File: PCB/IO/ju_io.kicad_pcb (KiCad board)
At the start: 2 copper layers, 30 x 65 mm, 17 parts, among them J1 Conn_01x05, J2 Conn_01x05, J3 Conn_01x05, J4 Conn_01x05, J5 Conn_01x03, J6 Conn_01x03, U1 PiPico_No_SWD

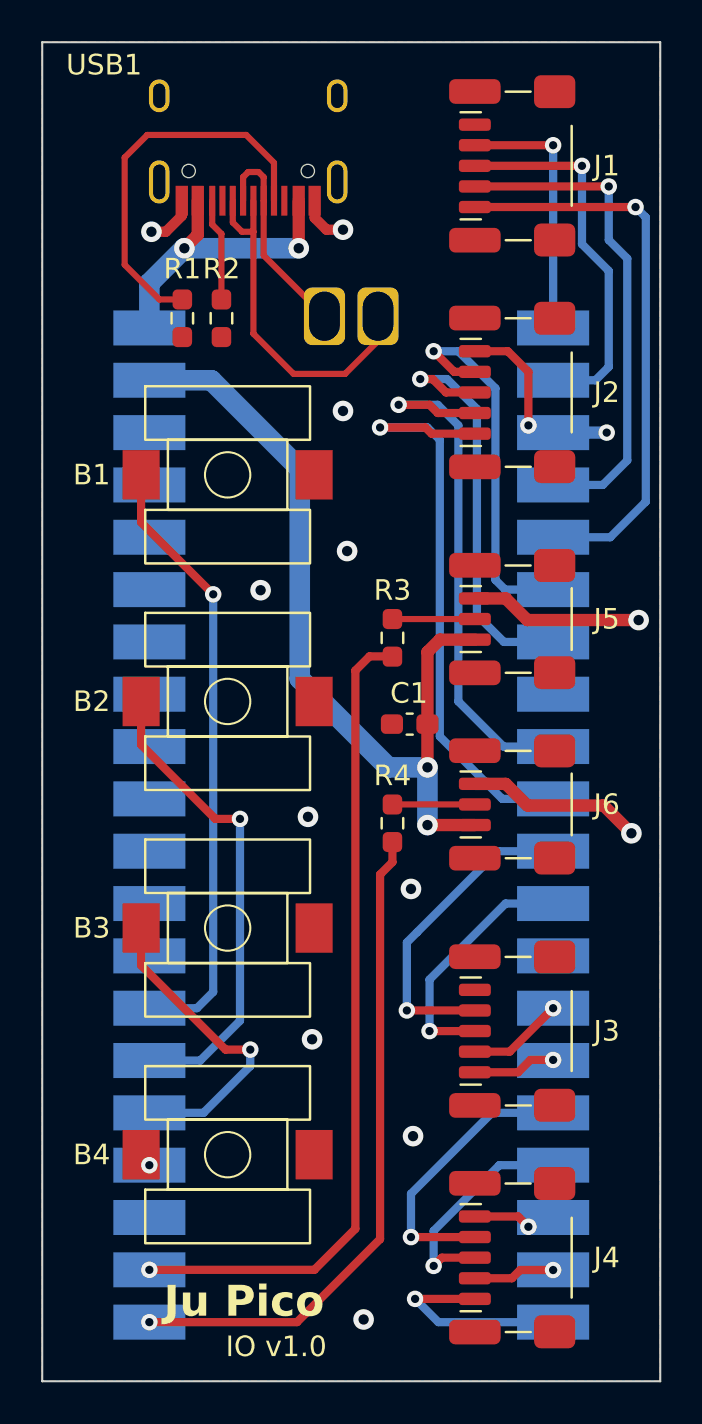
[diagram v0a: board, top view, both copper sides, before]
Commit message: PCBs of v1.1
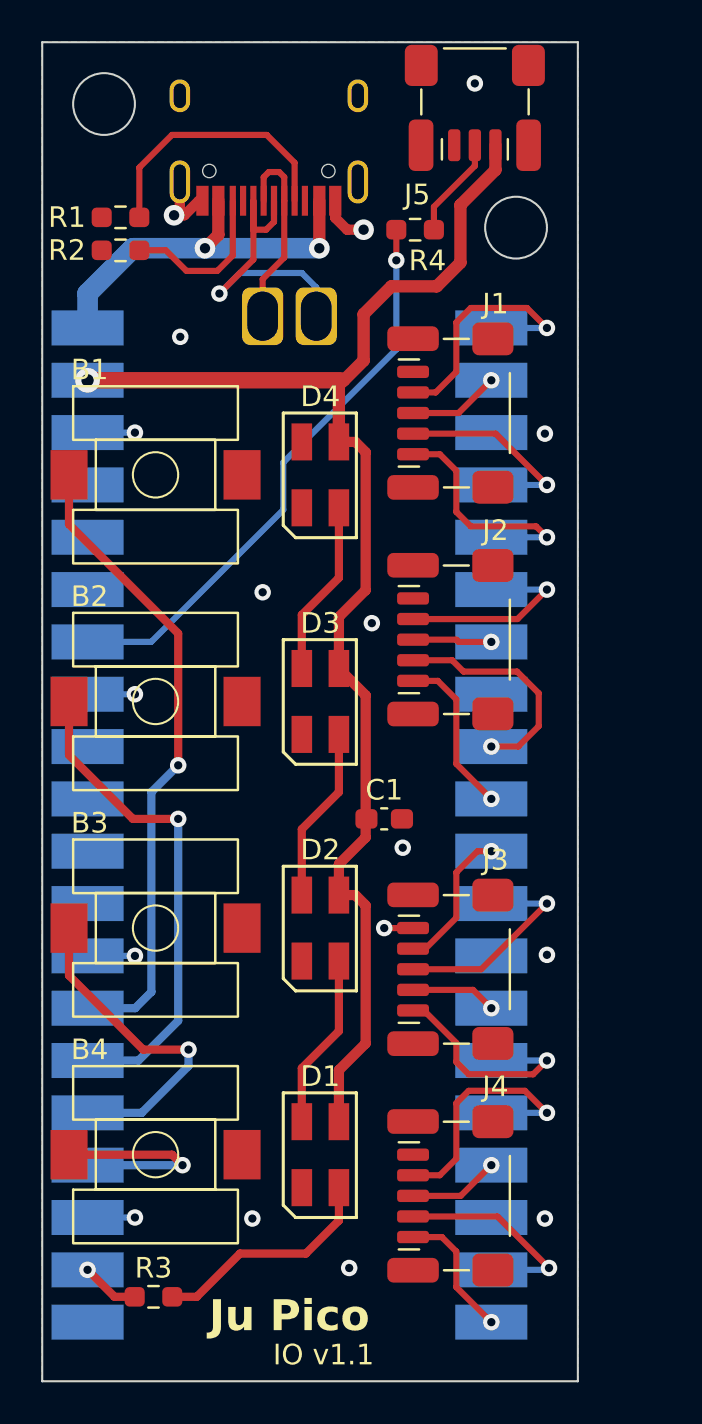
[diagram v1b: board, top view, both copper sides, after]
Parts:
- removed J6: Conn_01x03, ju_io:SH1.0_3P
- added D1: WS2812B_Unified, ju_io:WS2812B-2835, F.Cu at (138.6, 121.7)
- added D2: WS2812B_Unified, ju_io:WS2812B-2835, F.Cu at (138.6, 110.7)
- added D3: WS2812B_Unified, ju_io:WS2812B-2835, F.Cu at (138.6, 99.7)
- added D4: WS2812B_Unified, ju_io:WS2812B-2835, F.Cu at (138.6, 88.7)
- U1: footprint ju_io:RPi_Pico_SMD_Pins_No_SWD -> ju_io:RPi_Pico_SMD_Pins_No_SWD_No_Text
- moved R3 34.0 mm to (130.5, 128.6), turned to 0 degrees
- moved R4 28.8 mm to (143.2, 76.8), turned to 0 degrees
- moved J5 25.1 mm to (146.1, 70.7), turned to 180 degrees
- moved J1 12.4 mm to (145.1, 85.7)
- moved J2 12.4 mm to (145.1, 96.7)
- moved R2 5.91 mm to (128.9, 77.8), turned to 180 degrees
- moved R1 5.75 mm to (128.9, 76.2), turned to 180 degrees
- moved C1 4.76 mm to (141.7, 105.4), turned to 0 degrees
- moved J3 4.24 mm to (145.1, 112.7)
- moved J4 4.24 mm to (145.1, 123.7)
- moved B1 3.50 mm to (130.6, 88.7)
- moved B2 3.50 mm to (130.6, 99.7)
- moved B3 3.50 mm to (130.6, 110.7)
- moved B4 3.50 mm to (130.6, 121.7)
- moved U1 3.00 mm to (137.1, 105.7)
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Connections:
- R3 pad 2: Net-(J5-Pin_2) -> Net-(D1-In)
- R4 pad 1: Net-(U1-GPIO16) -> Net-(U1-GPIO28_ADC2)
- R4 pad 2: Net-(J6-Pin_2) -> Net-(J5-Pin_2)
- U1 pad 21: Net-(U1-GPIO16) -> unconnected-(U1-GPIO16-Pad21)
- U1 pad 34: unconnected-(U1-GPIO28_ADC2-Pad34) -> Net-(U1-GPIO28_ADC2)
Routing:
- net Net-(U1-GPIO17): track 40.0 -> 2.83 mm
- net Net-(U1-GPIO16): track 32.4 -> 0.00 mm, vias 1 -> 0
- net Net-(U1-GPIO28_ADC2): track 0.00 -> 28.0 mm, vias 0 -> 1
- net +5V: track 40.5 -> 68.4 mm, vias 2 -> 1
- net Net-(J2-Pin_1): track 29.0 -> 8.01 mm
- net Net-(J2-Pin_3): track 20.5 -> 3.85 mm
- net GND: track 33.0 -> 16.4 mm, vias 15 -> 17
- net Net-(J1-Pin_1): track 27.5 -> 12.0 mm
- net Net-(J2-Pin_2): track 26.1 -> 11.1 mm
- net Net-(J1-Pin_2): track 24.3 -> 10.2 mm
- net Net-(J1-Pin_3): track 18.5 -> 4.46 mm
- net Net-(D1-In): track 0.00 -> 11.2 mm
- net Net-(B4-A): track 0.00 -> 10.3 mm
- net Net-(J2-Pin_4): track 18.5 -> 9.79 mm
- net Net-(D3-Out): track 0.00 -> 8.55 mm
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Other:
- board size 30 x 65 mm -> 26 x 65 mm
- board text added: "IO v1.1"
- board text removed: "IO v1.0"
- board text removed: "JLCJLCJLCJLC"
